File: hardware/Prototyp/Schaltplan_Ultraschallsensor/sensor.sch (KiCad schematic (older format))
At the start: 14 parts, among them U2 TLC272

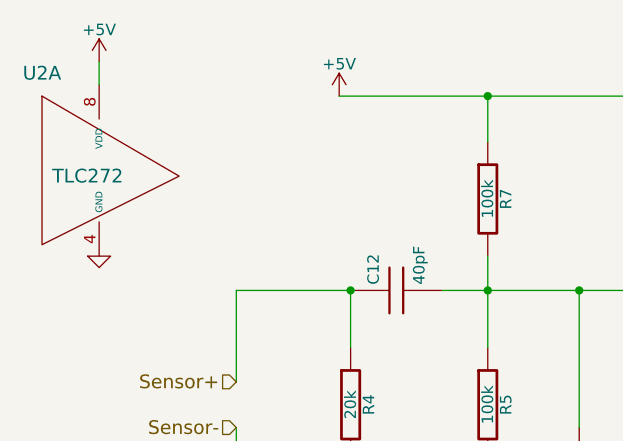
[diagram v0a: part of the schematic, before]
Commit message: Layout
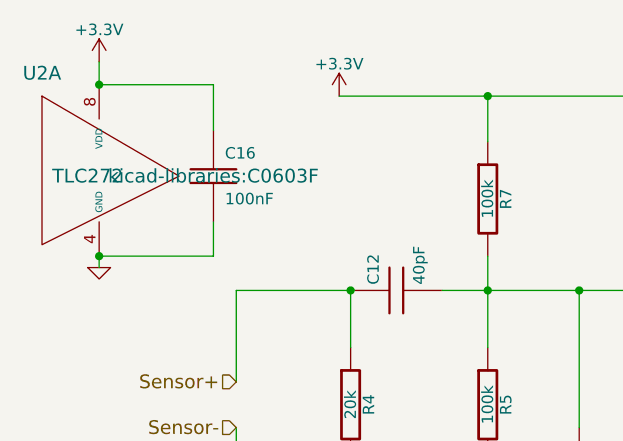
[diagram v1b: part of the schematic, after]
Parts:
- added C16: 100nF, kicad-libraries:C0603F, symbol C
- D2: footprint kicad-libraries:DO-214AA -> kicad-libraries:SOD-123
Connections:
- net GND: now also C16.2
- net +5V renamed +3V3
- net +3V3: now also C16.1
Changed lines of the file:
@@
 Connection ~ 5700 3850
 $Comp
-L GND #PWR027
+L GND #PWR020
 U 1 1 5A70B233
 P 2200 4100
-F 0 "#PWR027" H 2200 4100 30  0001 C CNN
+F 0 "#PWR020" H 2200 4100 30  0001 C CNN
 F 1 "GND" H 2200 4030 30  0001 C CNN
 F 2 "" H 2200 4100 60  0000 C CNN
 F 3 "" H 2200 4100 60  0000 C CNN
 	1    2200 4100
-	1    0    0    -1
-$EndComp
-$Comp
-L +5V #PWR028
-U 1 1 5A70745C
-P 2150 1050
-F 0 "#PWR028" H 2150 900 50  0001 C CNN
-F 1 "+5V" H 2150 1190 50  0000 C CNN
-F 2 "" H 2150 1050 50  0001 C CNN
-F 3 "" H 2150 1050 50  0001 C CNN
-	1    2150 1050
 	1    0    0    -1
 $EndComp
@@
 	1    0    0    -1
 $EndComp
-$Comp
-L GND #PWR029
-U 1 1 5A711570
-P 1100 1750
-F 0 "#PWR029" H 1100 1750 30  0001 C CNN
-F 1 "GND" H 1100 1680 30  0001 C CNN
-F 2 "" H 1100 1750 60  0000 C CNN
-F 3 "" H 1100 1750 60  0000 C CNN
-	1    1100 1750
-	1    0    0    -1
-$EndComp
-$Comp
-L +5V #PWR030
-U 1 1 5A7115A2
-P 1100 900
-F 0 "#PWR030" H 1100 750 50  0001 C CNN
-F 1 "+5V" H 1100 1040 50  0000 C CNN
-F 2 "" H 1100 900 50  0001 C CNN
-F 3 "" H 1100 900 50  0001 C CNN
-	1    1100 900
-	1    0    0    -1
-$EndComp
 Wire Wire Line
 	7300 3850 7300 3000
-Wire Wire Line
-	1100 1000 1100 900
 $Comp
 L ZENER D2
@@
 F 0 "D2" H 3200 2800 50  0000 C CNN
 F 1 "ZENER" H 3200 2600 50  0000 C CNN
-F 2 "kicad-libraries:DO-214AA" H 3200 2700 50  0001 C CNN
+F 2 "kicad-libraries:SOD-123" H 3200 2700 50  0001 C CNN
 F 3 "" H 3200 2700 50  0000 C CNN
 	1    3200 2700
@@
 	2800 2650 2800 3850
 Connection ~ 2800 3850
+$Comp
+L C C16
+U 1 1 5A780601
+P 1600 1400
+F 0 "C16" H 1650 1500 50  0000 L CNN
+F 1 "100nF" H 1650 1300 50  0000 L CNN
+F 2 "kicad-libraries:C0603F" H 1600 1400 60  0000 C CNN
+F 3 "" H 1600 1400 60  0000 C CNN
+	1    1600 1400
+	1    0    0    -1
+$EndComp
+$Comp
+L +3.3V #PWR021
+U 1 1 5A780C6E
+P 2150 1050
+F 0 "#PWR021" H 2150 900 50  0001 C CNN
+F 1 "+3.3V" H 2150 1190 50  0000 C CNN
+F 2 "" H 2150 1050 50  0001 C CNN
+F 3 "" H 2150 1050 50  0001 C CNN
+	1    2150 1050
+	1    0    0    -1
+$EndComp
+Wire Wire Line
+	1100 1000 1600 1000
+Wire Wire Line
+	1600 1000 1600 1200
+Wire Wire Line
+	1100 1750 1600 1750
+Wire Wire Line
+	1600 1750 1600 1600
+Wire Wire Line
+	1100 1750 1100 1800
+Connection ~ 1100 1000
+Connection ~ 1100 1750
+$Comp
+L GND #PWR022
+U 1 1 5A78FDAF
+P 1100 1800
+F 0 "#PWR022" H 1100 1800 30  0001 C CNN
+F 1 "GND" H 1100 1730 30  0001 C CNN
+F 2 "" H 1100 1800 60  0000 C CNN
+F 3 "" H 1100 1800 60  0000 C CNN
+	1    1100 1800
+	1    0    0    -1
+$EndComp
+$Comp
+L +3.3V #PWR023
+U 1 1 5A792C08
+P 1100 900
+F 0 "#PWR023" H 1100 750 50  0001 C CNN
+F 1 "+3.3V" H 1100 1040 50  0000 C CNN
+F 2 "" H 1100 900 50  0001 C CNN
+F 3 "" H 1100 900 50  0001 C CNN
+	1    1100 900
+	1    0    0    -1
+$EndComp
+Wire Wire Line
+	1100 900  1100 1000
 $EndSCHEMATC

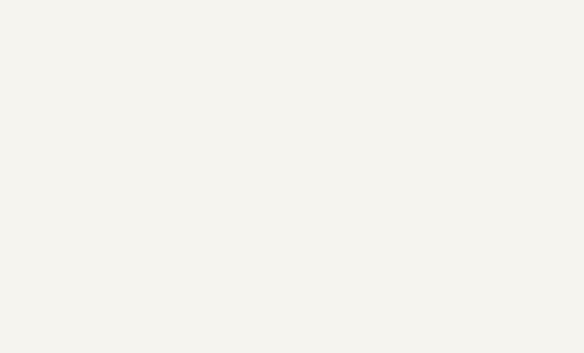
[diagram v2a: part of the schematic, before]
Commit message: Befestigungen
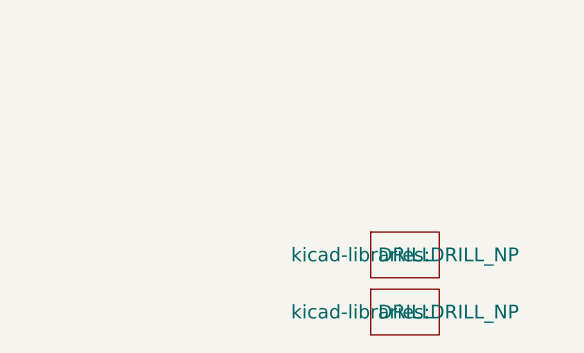
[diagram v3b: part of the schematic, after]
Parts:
- added U5, U6: DRILL, kicad-libraries:DRILL_NP, symbol DRILL
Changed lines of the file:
@@
 Wire Wire Line
 	1100 900  1100 1000
+$Comp
+L DRILL U6
+U 1 1 5A7AB1D9
+P 11050 6400
+F 0 "U6" H 11100 6450 60  0001 C CNN
+F 1 "DRILL" H 11050 6400 60  0000 C CNN
+F 2 "kicad-libraries:DRILL_NP" H 11050 6400 60  0000 C CNN
+F 3 "" H 11050 6400 60  0000 C CNN
+	1    11050 6400
+	1    0    0    -1
+$EndComp
+$Comp
+L DRILL U5
+U 1 1 5A7AB2B7
+P 11050 6150
+F 0 "U5" H 11100 6200 60  0001 C CNN
+F 1 "DRILL" H 11050 6150 60  0000 C CNN
+F 2 "kicad-libraries:DRILL_NP" H 11050 6150 60  0000 C CNN
+F 3 "" H 11050 6150 60  0000 C CNN
+	1    11050 6150
+	1    0    0    -1
+$EndComp
 $EndSCHEMATC
